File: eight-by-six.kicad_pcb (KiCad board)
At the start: 2 copper layers, 171.4 x 171.4 mm, 108 parts, among them J1 Left, J2 Right, SW1 Key, SW10 Key, SW11 Key, SW12 Key, SW13 Key, SW14 Key, SW15 Key, SW16 Key, SW17 Key, SW18 Key, SW19 Key, SW2 Key, SW20 Key, SW21 Key, SW22 Key, SW23 Key, SW24 Key, SW25 Key, SW26 Key, SW27 Key, SW28 Key, SW29 Key, SW3 Key, SW30 Key, SW31 Key, SW32 Key, SW33 Key, SW34 Key, SW35 Key, SW36 Key, SW37 Key, SW38 Key, SW39 Key, SW4 Key, SW40 Key, SW41 Key, SW42 Key, SW43 Key, SW44 Key, SW45 Key, SW46 Key, SW47 Key, SW48 Key, SW5 Key, SW6 Key, SW7 Key, SW8 Key, SW9 Key

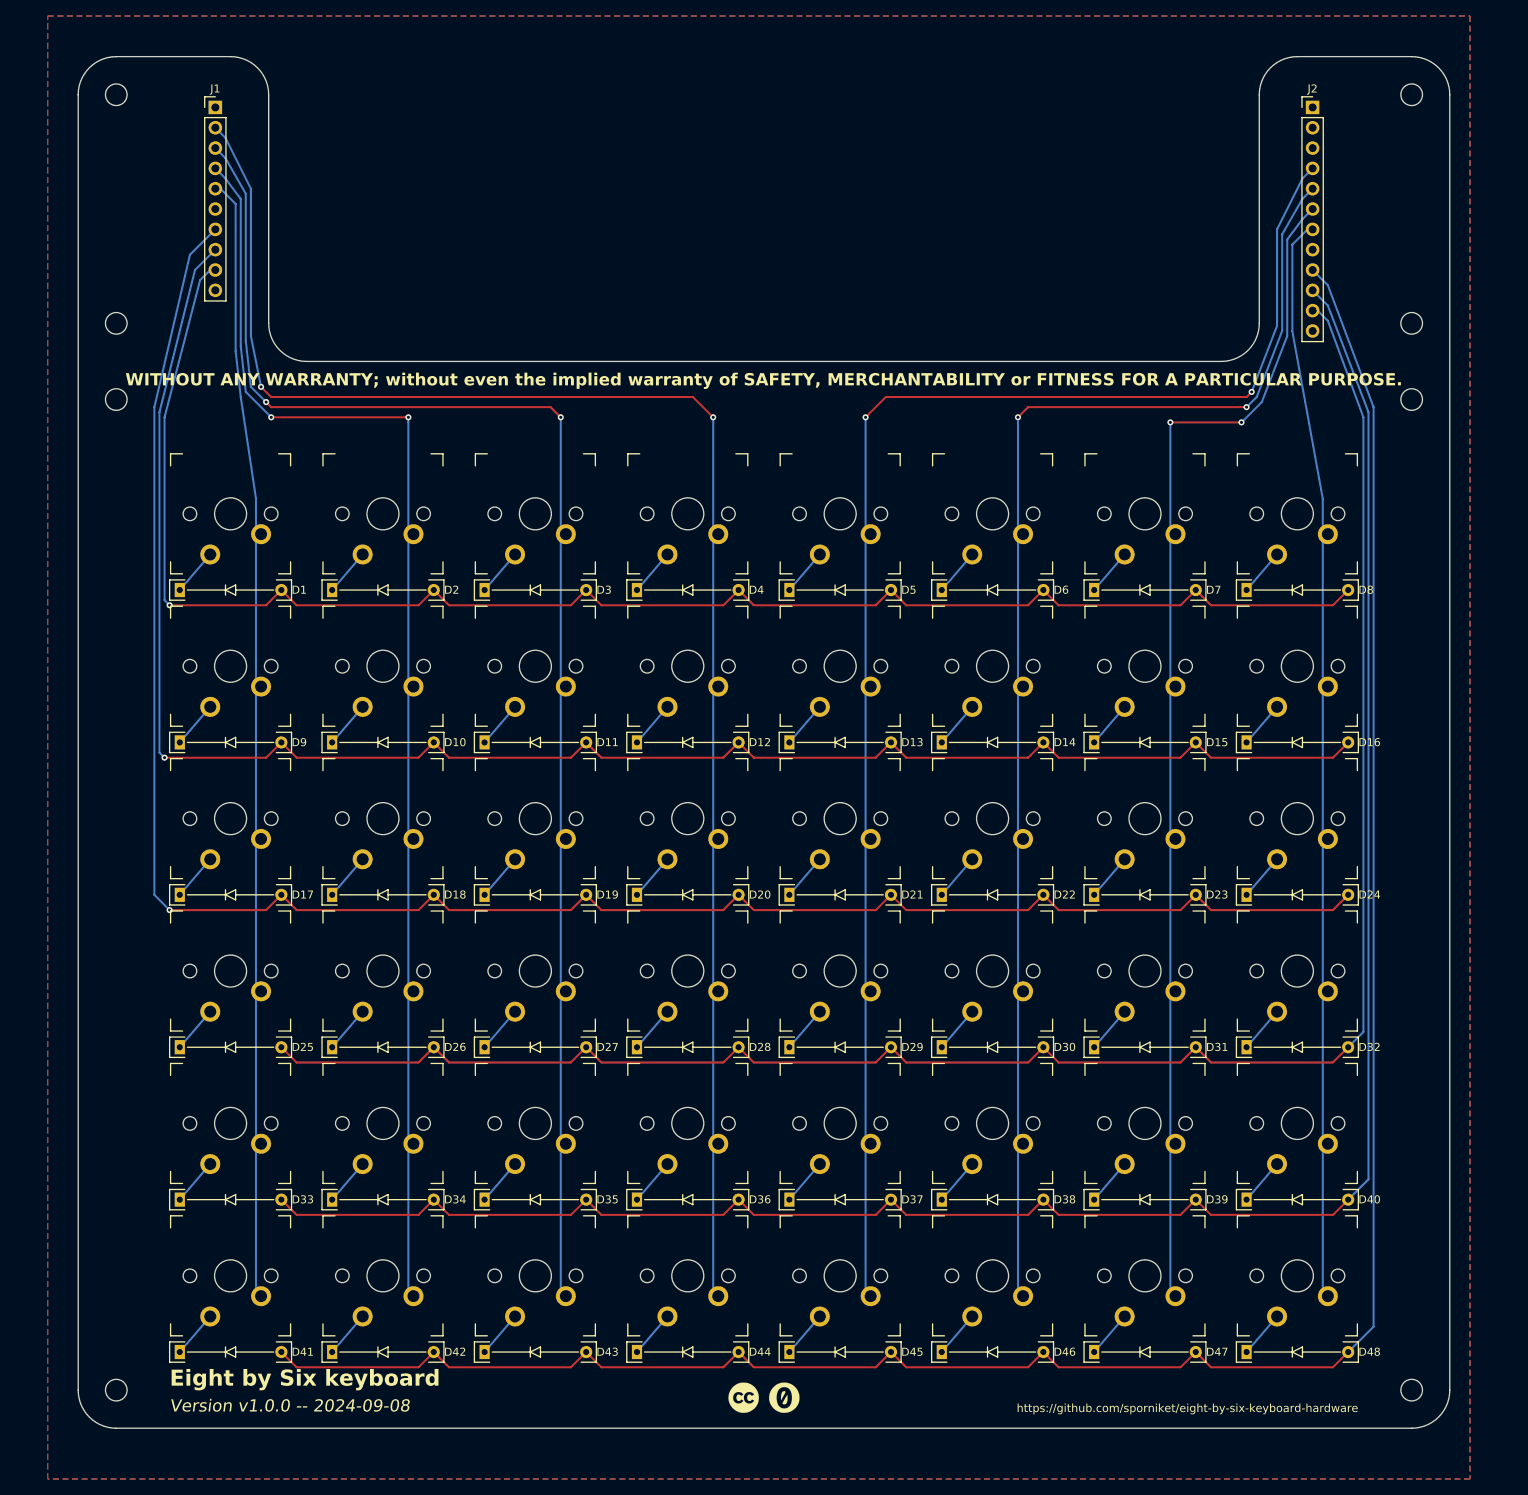
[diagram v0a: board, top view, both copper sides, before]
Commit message: Done all measurement and cuts
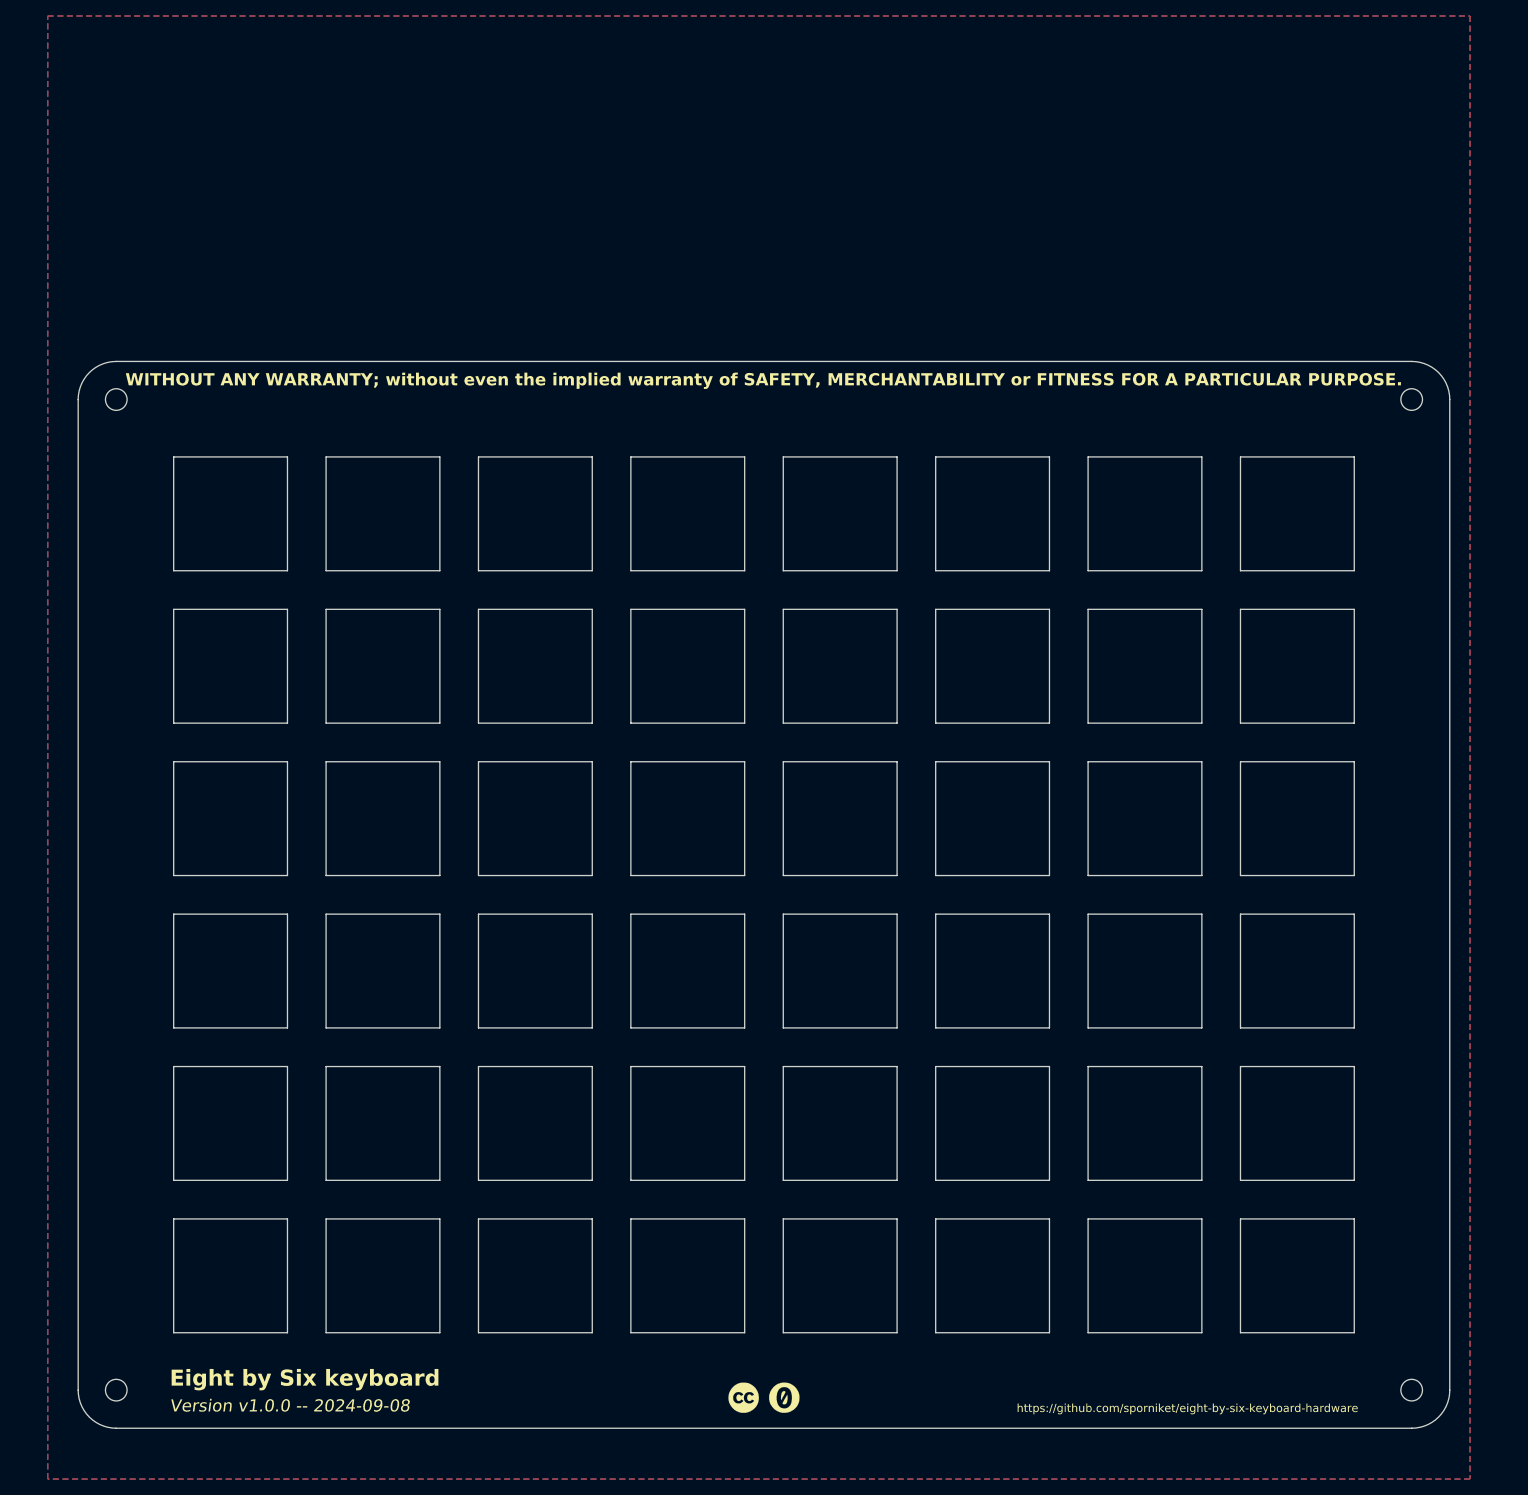
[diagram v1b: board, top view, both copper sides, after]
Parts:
- removed D1, D10, D11, D12, D13, D14, D15, D16, D17, D18, D19, D2, D20, D21, D22, D23, D24, D25, D26, D27, D28, D29, D3, D30, D31, D32, D33, D34, D35, D36, D37, D38, D39, D4, D40, D41, D42, D43, D44, D45, D46, D47, D48, D5, D6, D7, D8, D9: 1N4148, commons-passives_THT:Passive_THT_diode_W2.54mm_L12.70mm
- removed the H1 at (23.8, 81.0)
- removed the H2 at (23.8, 109.5)
- removed H5, H6: M2.5, MountingHole:MountingHole_2.7mm_M2.5
- removed J1: Left, Connector_PinHeader_2.54mm:PinHeader_1x10_P2.54mm_Vertical
- removed J2: Right, Connector_PinHeader_2.54mm:PinHeader_1x12_P2.54mm_Vertical
- removed SW1, SW10, SW11, SW12, SW13, SW14, SW15, SW16, SW17, SW18, SW19, SW2, SW20, SW21, SW22, SW23, SW24, SW25, SW26, SW27, SW28, SW29, SW3, SW30, SW31, SW32, SW33, SW34, SW35, SW36, SW37, SW38, SW39, SW4, SW40, SW41, SW42, SW43, SW44, SW45, SW46, SW47, SW48, SW5, SW6, SW7, SW8, SW9: Key, key-switches:SW_MX_THT
- renumbered H3 to H1, H4 to H2, H7 to H3, H8 to H4
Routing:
- net /r5: track 282.8 -> 0.00 mm
- net /r4: track 260.8 -> 0.00 mm
- net /r2: track 246.9 -> 0.00 mm, vias 1 -> 0
- net /r3: track 239.2 -> 0.00 mm
- net /r1: track 225.2 -> 0.00 mm, vias 1 -> 0
- net /c3: track 204.6 -> 0.00 mm, vias 2 -> 0
- net /r0: track 203.1 -> 0.00 mm, vias 1 -> 0
- net /c4: track 192.1 -> 0.00 mm, vias 2 -> 0
- net /c2: track 184.1 -> 0.00 mm, vias 2 -> 0
- net /c5: track 171.5 -> 0.00 mm, vias 2 -> 0
- net /c1: track 163.5 -> 0.00 mm, vias 2 -> 0
- net /c6: track 150.5 -> 0.00 mm, vias 2 -> 0
- net /c0: track 142.9 -> 0.00 mm
- net /c7: track 138.0 -> 0.00 mm
- net Net-(D9-K): track 5.85 -> 0.00 mm
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- added copper zone on B.Cu, net (none)
- added copper zone on F.Cu, net (none)
- removed copper zone on B.Cu, net GND
- removed copper zone on F.Cu, net GND
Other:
- board size 171.4 x 171.4 mm -> 171.4 x 133.4 mm
